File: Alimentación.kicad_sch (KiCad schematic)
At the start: 1 part, among them IC1 LDO40LPURY

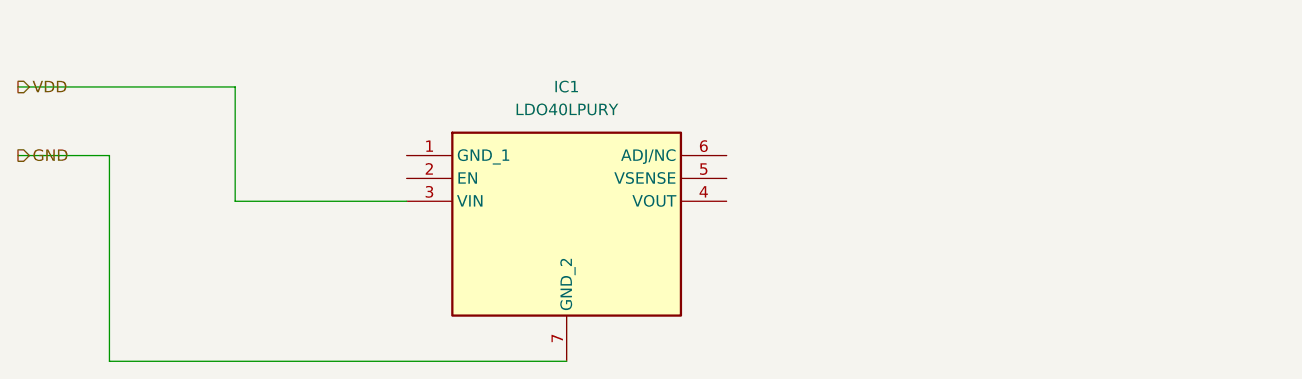
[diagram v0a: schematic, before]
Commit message: Add files via upload
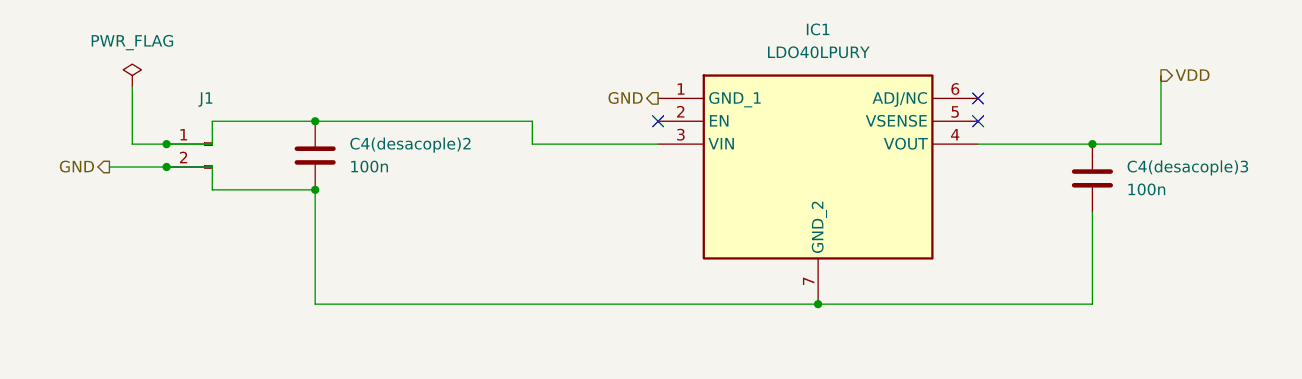
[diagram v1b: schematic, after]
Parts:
- added C4(desacople)2, C4(desacople)3: 100n, Capacitor_SMD:C_0805_2012Metric, symbol Device:C
- added J1: Conn_01x02_Pin, Connector_PinHeader_1.00mm:PinHeader_1x02_P1.00mm_Horizontal, symbol Connector:Conn_01x02_Pin
- IC1: footprint SON95P300X300X90-7N-D -> Package_DFN_QFN:DFN-6-1EP_3x3mm_P0.95mm_EP1.7x2.6mm; now left out of the parts list
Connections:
- net GND: now also IC1.1 (GND_1), C4(desacople)2.2, C4(desacople)3.2, J1.2 (Pin_2)
- net VDD: now also IC1.4 (VOUT), C4(desacople)3.1; no longer IC1.3 (VIN)
- new net: C4(desacople)2.1, IC1.3 (VIN), J1.1 (Pin_1)
- no-connect marks 0 -> 3
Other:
- moved on the sheet: IC1
